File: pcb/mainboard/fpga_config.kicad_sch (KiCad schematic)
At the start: 27 parts, among them J6 FH12-8S-0.5SH, J7 MICRO_SD(TFC-WPAPR-08), J8 DNP, SW1 SW, SW2 SW, U3 XC7Z010-CLG400, U30 W25Q128JVP, X1 33.33MHz

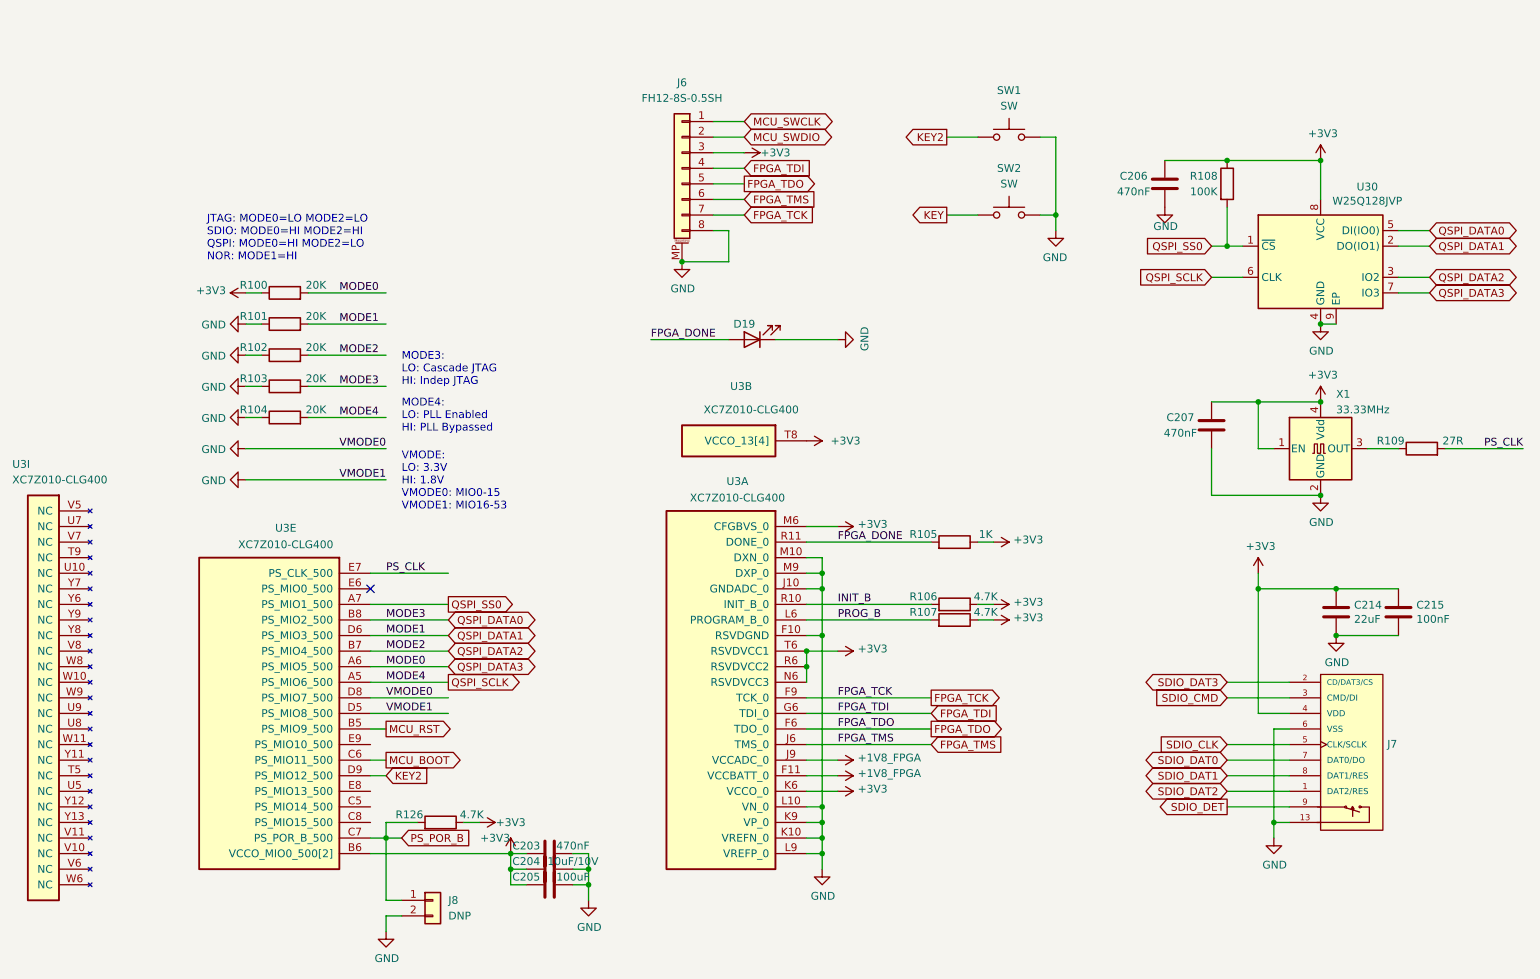
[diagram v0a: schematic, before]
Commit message: PCB r0p10 wip
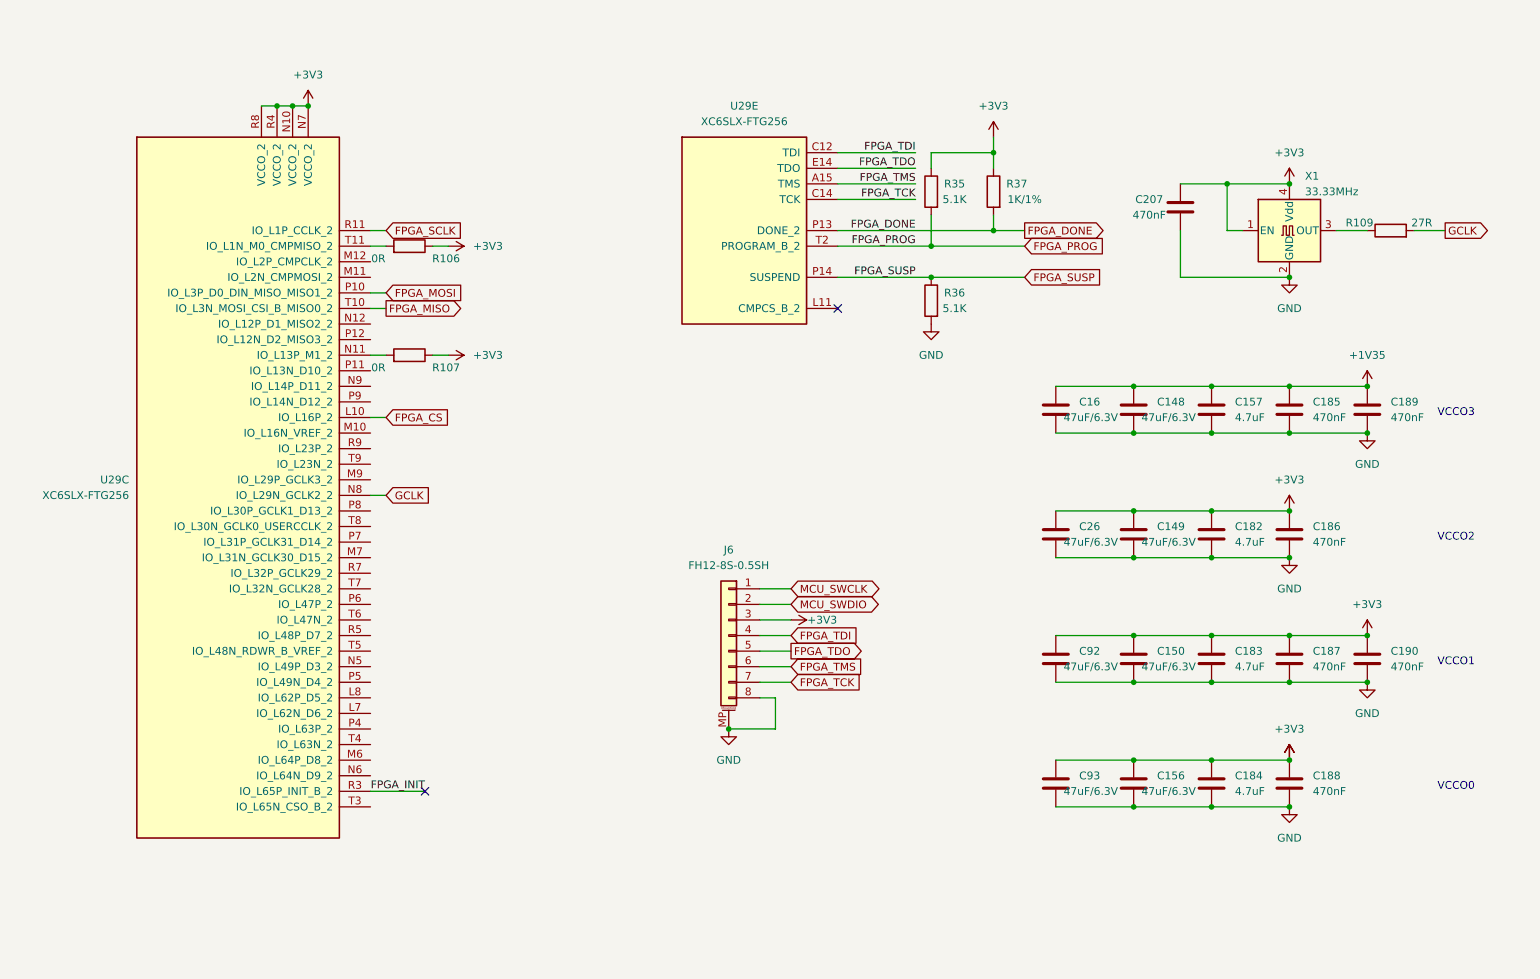
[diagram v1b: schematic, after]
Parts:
- removed C203, C206: 470nF, Capacitor_SMD:C_0402_1005Metric, symbol Device:C
- removed C204: 10uF/10V, Capacitor_SMD:C_0603_1608Metric, symbol Device:C
- removed C205: 100uF, Capacitor_SMD:C_0805_2012Metric, symbol Device:C
- removed C214: 22uF, Capacitor_SMD:C_0603_1608Metric, symbol Device:C
- removed C215: 100nF, Capacitor_SMD:C_0402_1005Metric, symbol Device:C
- removed D19: LED GREEN, LED_SMD:LED_0603_1608Metric, symbol Device:LED
- removed J7: MICRO_SD(TFC-WPAPR-08), footprints:TFC-WPAPR-08, symbol symbols:MICRO_SD(TFC-WPAPR-08)
- removed J8: DNP, Connector_PinHeader_2.00mm:PinHeader_1x02_P2.00mm_Vertical, symbol Connector_Generic:Conn_01x02
- removed R100, R101, R102, R103, R104: 20K, Resistor_SMD:R_0402_1005Metric, symbol Device:R
- removed R105: 1K, Resistor_SMD:R_0402_1005Metric, symbol Device:R
- removed R108: 100K, Resistor_SMD:R_0402_1005Metric, symbol Device:R
- removed R126: 4.7K, Resistor_SMD:R_0402_1005Metric, symbol Device:R
- removed SW1, SW2: SW, Button_Switch_SMD:Panasonic_EVQPUL_EVQPUC, symbol Switch:SW_Push
- removed U3: XC7Z010-CLG400, Package_BGA:Xilinx_CLG400, symbol symbols:XC7Z007S-CLG400
- removed U30: W25Q128JVP, Package_SON:WSON-8-1EP_6x5mm_P1.27mm_EP3.4x4mm, symbol Memory_Flash:W25Q32JVZP
- added C148, C149, C150, C156, C16, C26, C92, C93: 47uF/6.3V, Capacitor_SMD:C_0603_1608Metric, symbol Device:C
- added C157, C182, C183, C184: 4.7uF, Capacitor_SMD:C_0402_1005Metric, symbol Device:C
- added C185, C186, C187, C188, C189, C190: 470nF, Capacitor_SMD:C_0402_1005Metric, symbol Device:C
- added R35, R36: 5.1K, Resistor_SMD:R_0402_1005Metric, symbol Device:R
- added R37: 1K/1%, Resistor_SMD:R_0402_1005Metric, symbol Device:R
- added U29: XC6SLX-FTG256, symbol symbols:XC6SLX-FTG256
- R106, R107: value 4.7K -> 0R; Ref.Price (none) -> 0.0006
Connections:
- net +3V3: now also C149.1, C150.1, C156.1, C182.1, C183.1, C184.1, C186.1, C187.1, C188.1, C190.1, C26.1, C92.1, C93.1, R35.1, R37.1, U29.N10 (VCCO_2), U29.N7 (VCCO_2), U29.R4 (VCCO_2), U29.R8 (VCCO_2)
- net FPGA_DONE: now also R37.2, U29.P13 (DONE_2)
- net FPGA_TCK: now also U29.C14 (TCK)
- net FPGA_TDI: now also U29.C12 (TDI)
- net FPGA_TDO: now also U29.E14 (TDO)
- net FPGA_TMS: now also U29.A15 (TMS)
- net GND: now also C148.2, C149.2, C150.2, C156.2, C157.2, C16.2, C182.2, C183.2, C184.2, C185.2, C186.2, C187.2, C188.2, C189.2, C190.2, C26.2, C92.2, C93.2, R36.2
- net INIT_B: no longer names the net of R106.2
- net INIT_B: now also U29.T11 (IO_L1N_M0_CMPMISO_2)
- net PROG_B: no longer names the net of R107.2
- net PROG_B: now also U29.N11 (IO_L13P_M1_2)
- net PS_CLK renamed GCLK
- net GCLK: now also U29.N8 (IO_L29N_GCLK2_2)
- new net +1V35: C148.1, C157.1, C16.1, C185.1, C189.1
- new net FPGA_CS: U29.L10 (IO_L16P_2)
- new net FPGA_INIT: U29.R3 (IO_L65P_INIT_B_2)
- new net FPGA_MISO: U29.T10 (IO_L3N_MOSI_CSI_B_MISO0_2)
- new net FPGA_MOSI: U29.P10 (IO_L3P_D0_DIN_MISO_MISO1_2)
- new net FPGA_PROG: R35.2, U29.T2 (PROGRAM_B_2)
- new net FPGA_SCLK: U29.R11 (IO_L1P_CCLK_2)
- new net FPGA_SUSP: R36.1, U29.P14 (SUSPEND)
- no-connect marks 1 -> 2
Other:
- note added: "VCCO0"
- note added: "VCCO1"
- note added: "VCCO2"
- note added: "VCCO3"
- note removed: "JTAG: MODE0=LO MODE2=LO SDIO: MODE0=HI MODE2=HI QSPI: MODE0=HI MODE2=LO NOR: MODE1=HI"
- note removed: "MODE3: LO: Cascade JTAG HI: Indep JTAG"
- note removed: "MODE4: LO: PLL Enabled HI: PLL Bypassed"
- note removed: "VMODE: LO: 3.3V HI: 1.8V VMODE0: MIO0-15 VMODE1: MIO16-53"
- moved on the sheet: C207, J6, R109, X1

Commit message: PCB r0p10
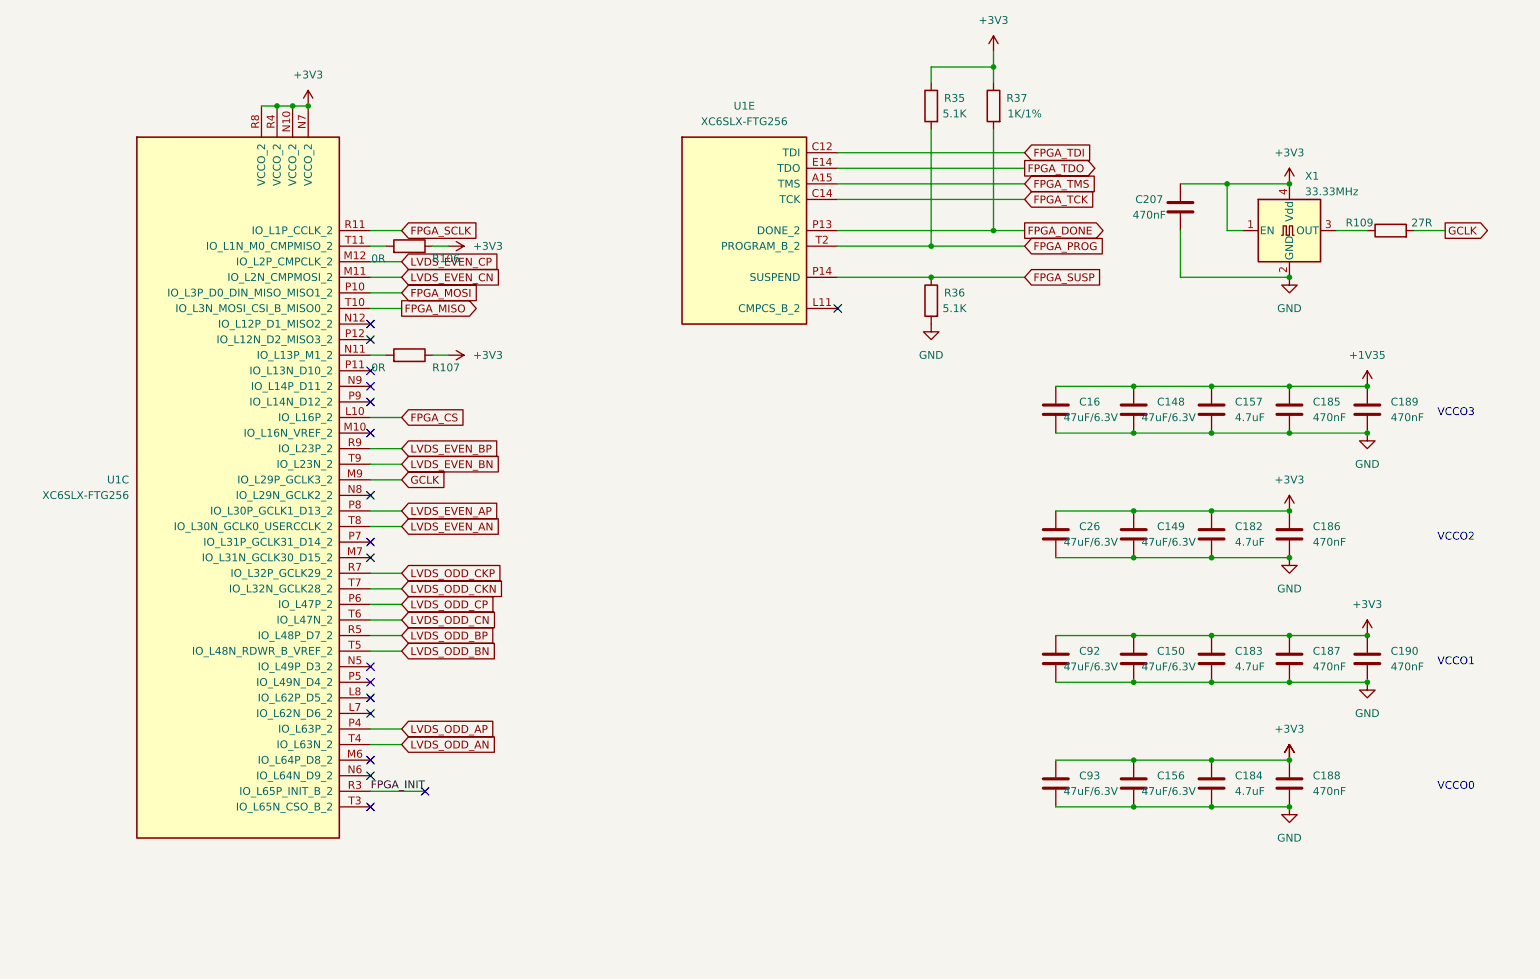
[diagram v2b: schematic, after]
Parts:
- removed J6: FH12-8S-0.5SH, Connector_FFC-FPC:Hirose_FH12-8S-0.5SH_1x08-1MP_P0.50mm_Horizontal, symbol Connector_Generic_MountingPin:Conn_01x08_MountingPin
- U1: renamed from U29; footprint (none) -> footprints:Xilinx_FTG256
- X1: footprint Crystal:Crystal_SMD_3225-4Pin_3.2x2.5mm -> Oscillator:Oscillator_SMD_Abracon_ASE-4Pin_3.2x2.5mm
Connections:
- net GCLK: now also U1.M9 (IO_L29P_GCLK3_2); no longer U1.N8 (IO_L29N_GCLK2_2)
- net LVDS_EVEN_CN: now reaches U1.M11 (IO_L2N_CMPMOSI_2)
- net LVDS_EVEN_CP: now reaches U1.M12 (IO_L2P_CMPCLK_2)
- net LVDS_ODD_AP: now reaches U1.P4 (IO_L63P_2)
- net LVDS_ODD_CP: now reaches U1.P6 (IO_L47P_2)
- net LVDS_EVEN_AP: now reaches U1.P8 (IO_L30P_GCLK1_D13_2)
- net LVDS_ODD_BP: now reaches U1.R5 (IO_L48P_D7_2)
- net LVDS_ODD_CKP: now reaches U1.R7 (IO_L32P_GCLK29_2)
- net LVDS_EVEN_BP: now reaches U1.R9 (IO_L23P_2)
- net LVDS_ODD_AN: now reaches U1.T4 (IO_L63N_2)
- net LVDS_ODD_BN: now reaches U1.T5 (IO_L48N_RDWR_B_VREF_2)
- net LVDS_ODD_CN: now reaches U1.T6 (IO_L47N_2)
- net LVDS_ODD_CKN: now reaches U1.T7 (IO_L32N_GCLK28_2)
- net LVDS_EVEN_AN: now reaches U1.T8 (IO_L30N_GCLK0_USERCCLK_2)
- net LVDS_EVEN_BN: now reaches U1.T9 (IO_L23N_2)
- no-connect marks 2 -> 18
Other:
- moved on the sheet: R35, R37
